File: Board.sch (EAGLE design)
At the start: 26 parts, among them IC1 BUF634U, IC2 LM555D, Q1 35A/25V/8.5mΩ, Q2 35A/25V/8.5mΩ, Q3 35A/25V/8.5mΩ, X3 MSTBV4

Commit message: PCB work
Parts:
- added CRYSTAL: (no value), con-subd:F25VP
- added J1: RASPBERRYPI-40-PIN-GPIO_PTH_NO_SHROUD, SparkFun-Connectors:RASPBERRYPI-40-PIN-GPIO_PTH_NO_SHROUD
- added Q4: 220mA/50V/3.5Ω, SparkFun-DiscreteSemi:MOSFET-NCH-BSS138
- added R3: 1k, resistor:R-US_R1206
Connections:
- new net N$11: IC2.TR, Q4.D, R3.2
- net +5V: now also R3.1
- net GND: now also Q4.S
- net RAWPPS: now also Q4.G
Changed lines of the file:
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@@
 <part name="SUPPLY42" library="supply2" deviceset="+5V" device=""/>
 <part name="SUPPLY43" library="supply2" deviceset="GND" device=""/>
+<part name="CRYSTAL" library="con-subd" deviceset="F25" device="VP"/>
+<part name="J1" library="SparkFun-Connectors" deviceset="RASPBERRYPI-40-PIN-GPIO" device="_PTH_NO_SHROUD"/>
+<part name="Q4" library="SparkFun-DiscreteSemi" deviceset="MOSFET-NCH" device="-BSS138" value="220mA/50V/3.5Ω"/>
+<part name="R3" library="resistor" deviceset="R-US_" device="R1206" value="1k"/>
+<part name="SUPPLY44" library="supply2" deviceset="+5V" device=""/>
+<part name="SUPPLY45" library="supply2" deviceset="GND" device=""/>
 </parts>
 <sheets>
@@
 <instance part="SUPPLY34" gate="GND" x="83.82" y="60.96"/>
 <instance part="SUPPLY35" gate="+5V" x="83.82" y="73.66"/>
+<instance part="Q4" gate="NMOS" x="27.94" y="48.26"/>
+<instance part="R3" gate="G$1" x="30.48" y="58.42" rot="R270"/>
+<instance part="SUPPLY44" gate="+5V" x="30.48" y="66.04"/>
+<instance part="SUPPLY45" gate="GND" x="30.48" y="40.64"/>
 </instances>
 <busses>
@@
 <pinref part="C5" gate="G$1" pin="2"/>
 <pinref part="SUPPLY34" gate="GND" pin="GND"/>
+</segment>
+<segment>
+<pinref part="Q4" gate="NMOS" pin="S"/>
+<pinref part="SUPPLY45" gate="GND" pin="GND"/>
 </segment>
 </net>
@@
 <pinref part="C5" gate="G$1" pin="1"/>
 <pinref part="SUPPLY35" gate="+5V" pin="+5V"/>
+</segment>
+<segment>
+<pinref part="R3" gate="G$1" pin="1"/>
+<pinref part="SUPPLY44" gate="+5V" pin="+5V"/>
 </segment>
 </net>
@@
 <wire x1="129.54" y1="17.78" x2="124.46" y2="17.78" width="0.1524" layer="91"/>
 <label x="124.46" y="17.78" size="1.778" layer="95" rot="R180"/>
+</segment>
+<segment>
+<pinref part="Q4" gate="NMOS" pin="G"/>
+<wire x1="22.86" y1="45.72" x2="17.78" y2="45.72" width="0.1524" layer="91"/>
+<label x="17.78" y="45.72" size="1.778" layer="95" rot="R180"/>
 </segment>
 </net>
@@
 <pinref part="IC1" gate="G$1" pin="BW"/>
 <pinref part="R2" gate="G$1" pin="1"/>
+</segment>
+</net>
+<net name="N$11" class="0">
+<segment>
+<pinref part="IC2" gate="A" pin="TR"/>
+<wire x1="50.8" y1="53.34" x2="30.48" y2="53.34" width="0.1524" layer="91"/>
+<pinref part="Q4" gate="NMOS" pin="D"/>
+<pinref part="R3" gate="G$1" pin="2"/>
+<junction x="30.48" y="53.34"/>
 </segment>
 </net>
@@
 <instance part="SUPPLY40" gate="GND" x="53.34" y="50.8"/>
 <instance part="SUPPLY41" gate="+24V" x="73.66" y="83.82"/>
+<instance part="CRYSTAL" gate="-1" x="20.32" y="25.4"/>
 </instances>
 <busses>
@@
 </nets>
 </sheet>
+<sheet>
+<description>Raspberry Pi</description>
+<plain>
+</plain>
+<instances>
+<instance part="J1" gate="G$1" x="53.34" y="58.42"/>
+</instances>
+<busses>
+</busses>
+<nets>
+</nets>
+</sheet>

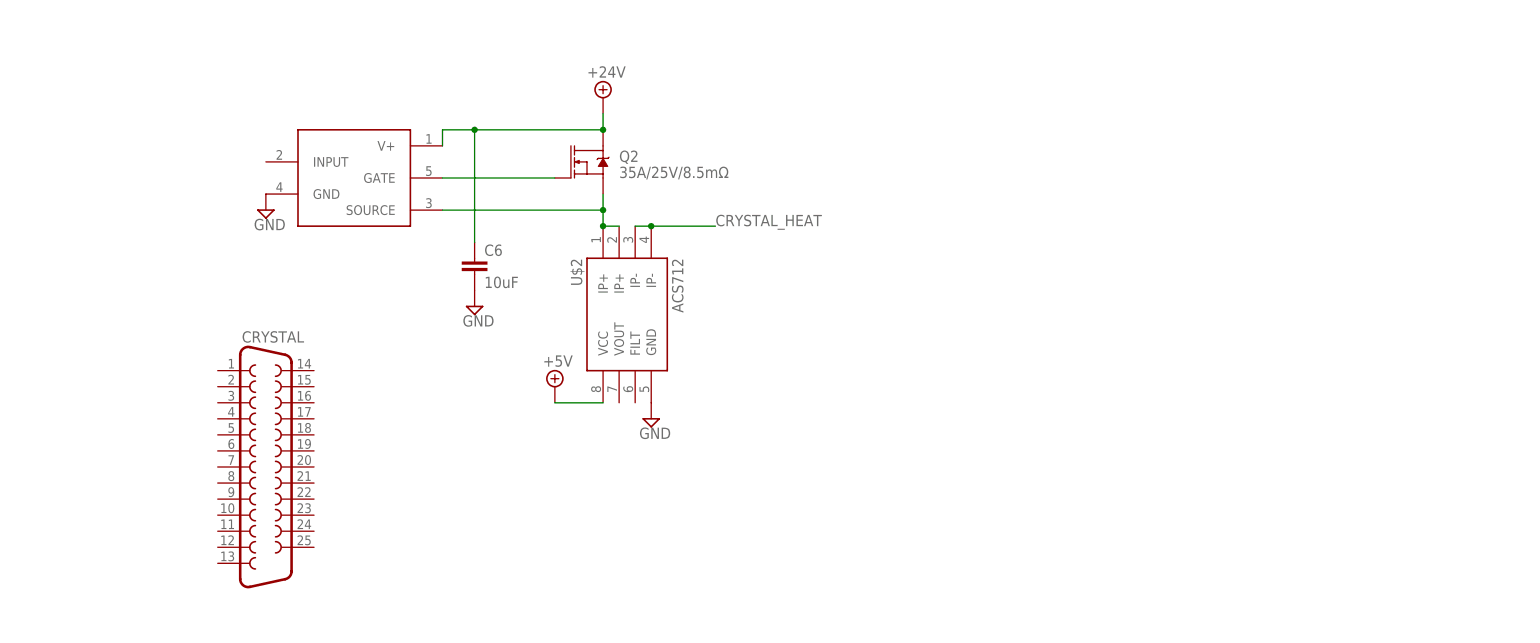
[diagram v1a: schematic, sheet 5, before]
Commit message: Adding crystal
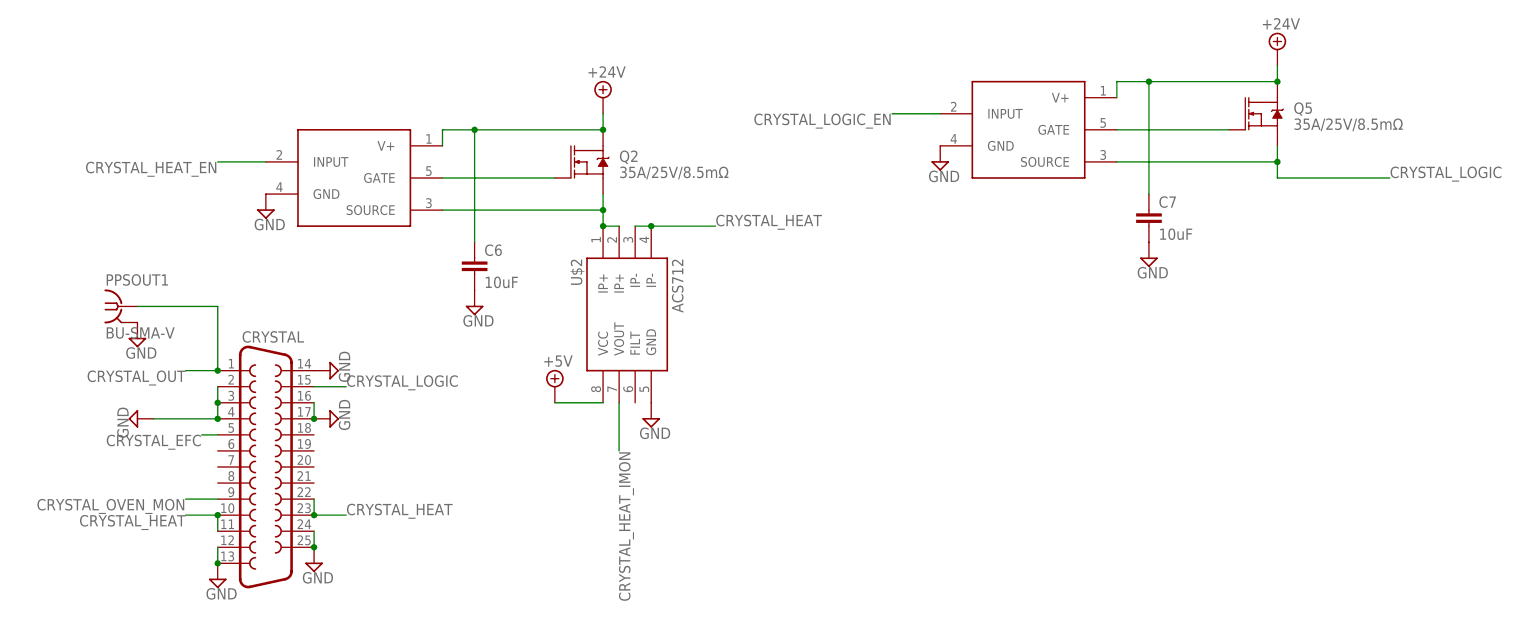
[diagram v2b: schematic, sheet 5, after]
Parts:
- added C7: 10uF, resistor:C-EUC1206
- added PPSOUT1: BU-SMA-V, con-coax:BU-SMA-V
- added Q5: 35A/25V/8.5mΩ, SparkFun-DiscreteSemi:MOSFET-NCH-FDD8780
- added U$8: MIC5014, FRC696:MIC5014
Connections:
- new net CRYSTAL_EFC: CRYSTAL.5
- new net CRYSTAL_HEAT_EN: U$5.INPUT
- new net CRYSTAL_HEAT_IMON: U$2.VOUT
- new net CRYSTAL_LOGIC: CRYSTAL.15, Q5.S, U$8.SOURCE
- new net CRYSTAL_LOGIC_EN: U$8.INPUT
- new net CRYSTAL_OUT: CRYSTAL.1, PPSOUT1.1
- new net CRYSTAL_OVEN_MON: CRYSTAL.9
- new net N$14: Q5.G, U$8.GATE
- net +24V: now also C7.1, Q5.D, U$8.V+
- net +5V: now also J1.5V@2, J1.5V@4
- net CRYSTAL_HEAT: now also CRYSTAL.10, CRYSTAL.11, CRYSTAL.22, CRYSTAL.23
- net GND: now also C7.2, CRYSTAL.12, CRYSTAL.13, CRYSTAL.14, CRYSTAL.16, CRYSTAL.17, CRYSTAL.2, CRYSTAL.24, CRYSTAL.25, CRYSTAL.3, CRYSTAL.4, J1.GND@14, J1.GND@20, J1.GND@25, J1.GND@30, J1.GND@34, J1.GND@39, J1.GND@6, J1.GND@9, PPSOUT1.2, U$8.GND
